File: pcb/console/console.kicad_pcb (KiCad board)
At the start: 2 copper layers, 80 x 60 mm, 5 parts, among them J1 Micro_SD_Card, SW1 CherryMX, SW2 CherryMX, U1 RP2040-ZERO

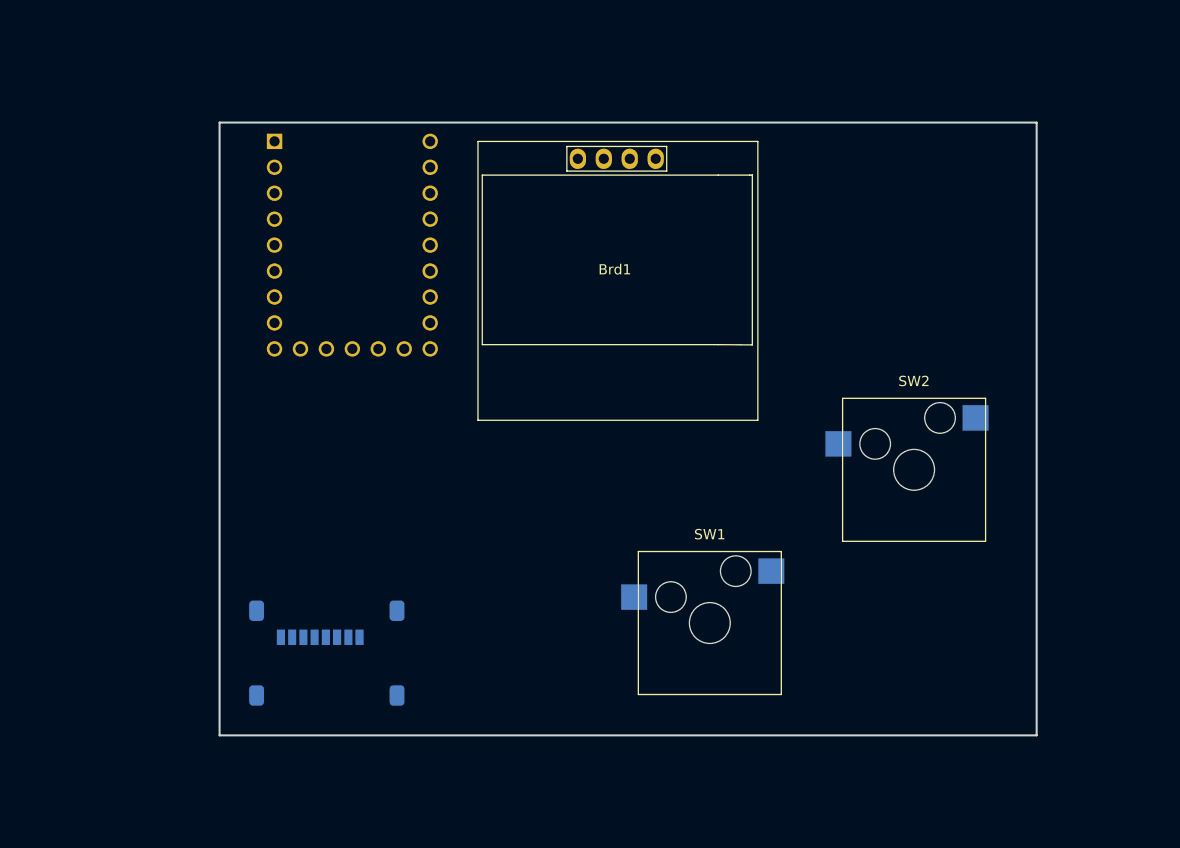
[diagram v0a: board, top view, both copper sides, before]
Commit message: ordered prototype
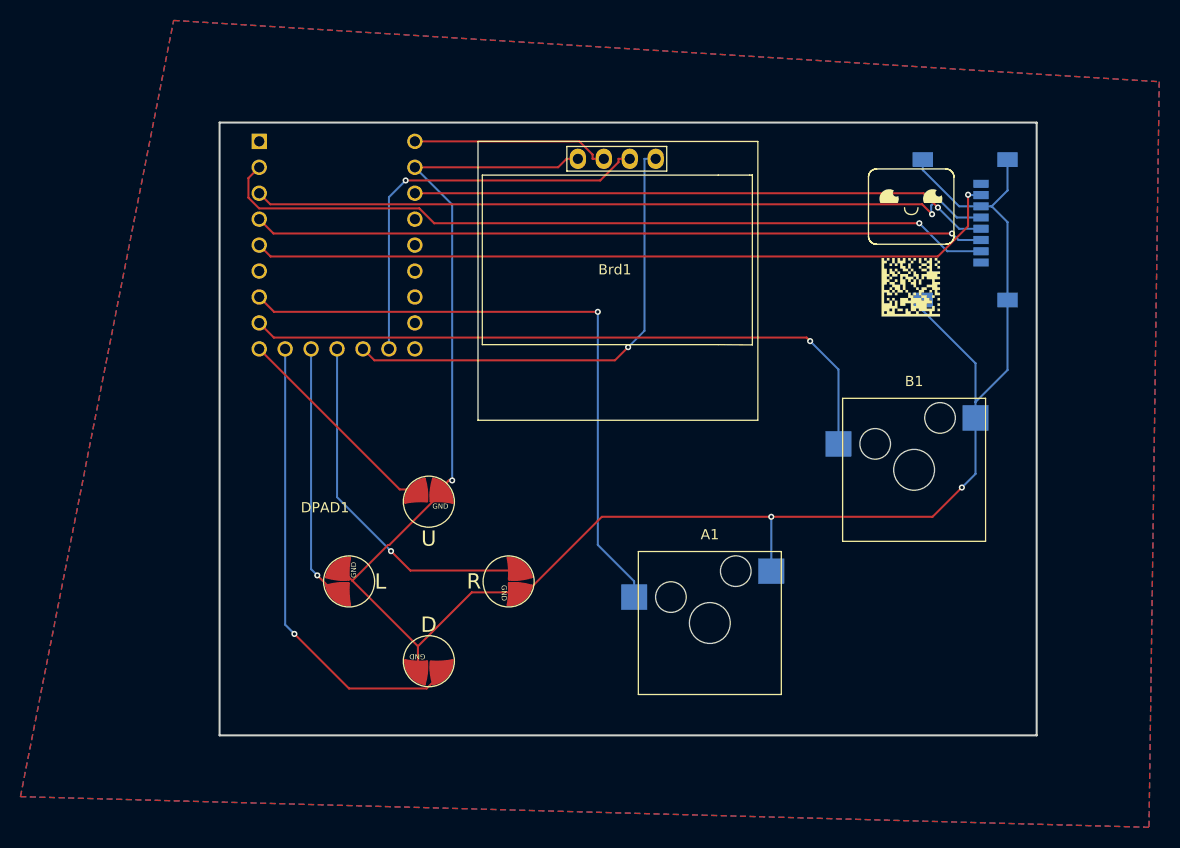
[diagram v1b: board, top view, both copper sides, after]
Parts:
- added DPAD1: GBC, gameboy-color:GBC DPAD, F.Cu at (184.5, 72.4)
- J1: footprint Connector_Card:microSD_HC_Molex_47219-2001 -> Connector_Card:microSD_HC_Wuerth_693072010801
- moved J1 75.3 mm to (237.0, 38.0), turned to 90 degrees
- moved U1 1.50 mm to (175.5, 39.5)
- renumbered SW1 to A1, SW2 to B1
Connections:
- A1 pad 1: unconnected-(SW1-Pad1) -> /A
- A1 pad 2: unconnected-(SW1-Pad2) -> GND
- B1 pad 1: unconnected-(SW2-Pad1) -> /B
- B1 pad 2: unconnected-(SW2-Pad2) -> GND
- Brd1 pad 1: unconnected-(Brd1-GND-Pad1) -> GND
- Brd1 pad 2: unconnected-(Brd1-VCC-Pad2) -> +5V
- Brd1 pad 3: unconnected-(Brd1-SCL-Pad3) -> /SCL0
- Brd1 pad 4: unconnected-(Brd1-SDA-Pad4) -> /SDA0
- J1 pad 2: unconnected-(J1-DAT3/CD-Pad2) -> /CS
- J1 pad 3: unconnected-(J1-CMD-Pad3) -> /MOSI
- J1 pad 4: unconnected-(J1-VDD-Pad4) -> +3.3V
- J1 pad 5: unconnected-(J1-CLK-Pad5) -> /SCLK
- J1 pad 6: unconnected-(J1-VSS-Pad6) -> GND
- J1 pad 7: unconnected-(J1-DAT0-Pad7) -> /MISO
- J1 pad 9: unconnected-(J1-SHIELD-Pad9) -> GND
- U1 pad 10: unconnected-(U1-GP9-Pad10) -> /DOWN
- U1 pad 11: unconnected-(U1-GP10-Pad11) -> /LEFT
- U1 pad 12: unconnected-(U1-GP11-Pad12) -> /RIGHT
- U1 pad 13: unconnected-(U1-GP12-Pad13) -> /SDA0
- U1 pad 14: unconnected-(U1-GP13-Pad14) -> /SCL0
- U1 pad 2: unconnected-(U1-GP1-Pad2) -> /CS
- U1 pad 21: unconnected-(U1-3V3-Pad21) -> +3.3V
- U1 pad 22: unconnected-(U1-GND-Pad22) -> GND
- U1 pad 23: unconnected-(U1-5V-Pad23) -> +5V
- U1 pad 3: unconnected-(U1-GP2-Pad3) -> /SCLK
- U1 pad 4: unconnected-(U1-GP3-Pad4) -> /MOSI
- U1 pad 5: unconnected-(U1-GP4-Pad5) -> /MISO
- U1 pad 7: unconnected-(U1-GP6-Pad7) -> /A
- U1 pad 8: unconnected-(U1-GP7-Pad8) -> /B
- U1 pad 9: unconnected-(U1-GP8-Pad9) -> /UP
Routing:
- net GND: track 0.00 -> 197.9 mm, vias 0 -> 3
- net /CS: track 0.00 -> 77.3 mm, vias 0 -> 1
- net /MISO: track 0.00 -> 75.5 mm, vias 0 -> 1
- net /SCLK: track 0.00 -> 73.3 mm, vias 0 -> 1
- net /MOSI: track 0.00 -> 71.5 mm, vias 0 -> 1
- net /B: track 0.00 -> 65.9 mm, vias 0 -> 1
- net /A: track 0.00 -> 63.2 mm, vias 0 -> 1
- net +3.3V: track 0.00 -> 56.9 mm, vias 0 -> 1
- net /SDA0: track 0.00 -> 47.2 mm, vias 0 -> 1
- net /DOWN: track 0.00 -> 45.4 mm, vias 0 -> 1
- net /SCL0: track 0.00 -> 40.2 mm, vias 0 -> 1
- net /RIGHT: track 0.00 -> 35.5 mm, vias 0 -> 1
- net /LEFT: track 0.00 -> 25.0 mm, vias 0 -> 1
- net /UP: track 0.00 -> 21.2 mm
- net +5V: track 0.00 -> 19.5 mm
- added copper zone on B.Cu, net GND
- added copper zone on F.Cu, net GND
